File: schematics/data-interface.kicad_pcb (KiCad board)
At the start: 4 copper layers, 30.1 x 69.9 mm, 18 parts, among them J2 USB_A, J5 Trigger Button Input Connector, Q1 2SC945, Q2 2SC945, Q3 2SC945, SW3 SW_Push, SW4 SW_DIP_x08

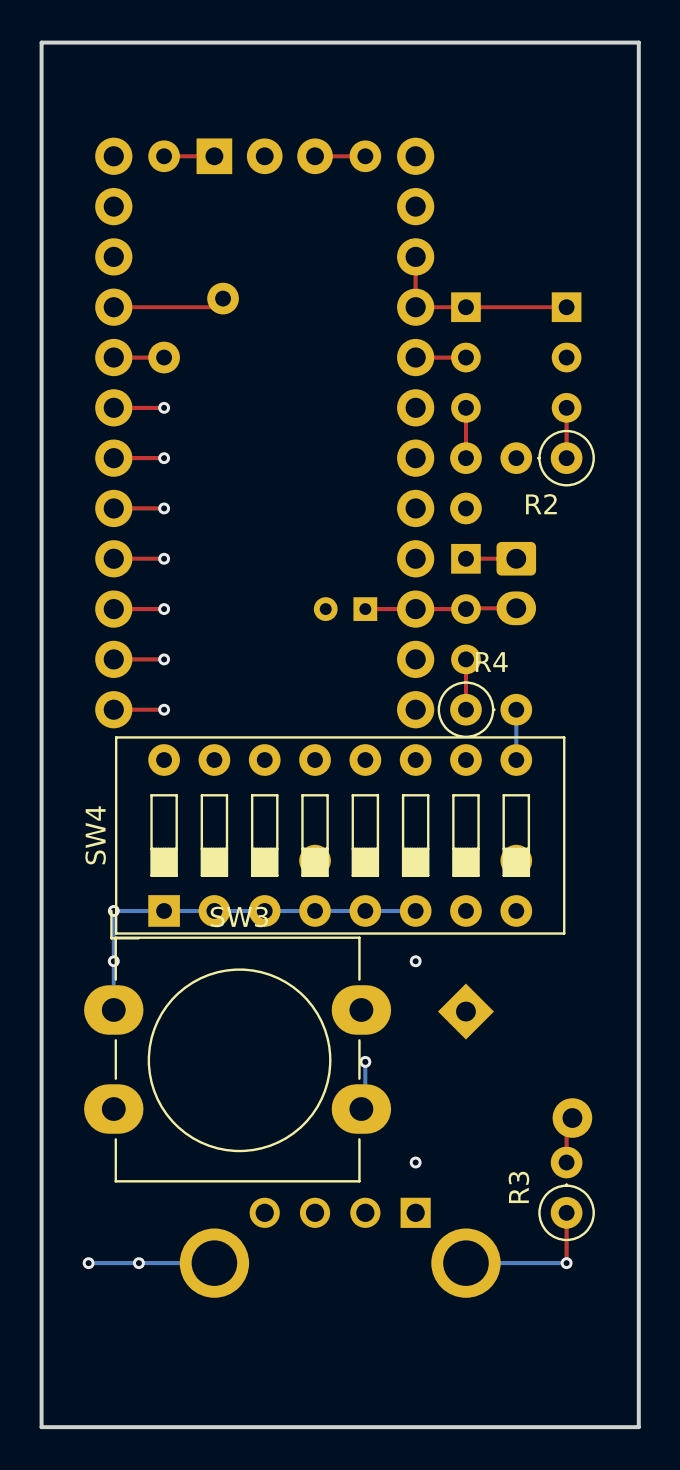
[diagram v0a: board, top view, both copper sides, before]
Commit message: Fixed minor errors in schematics
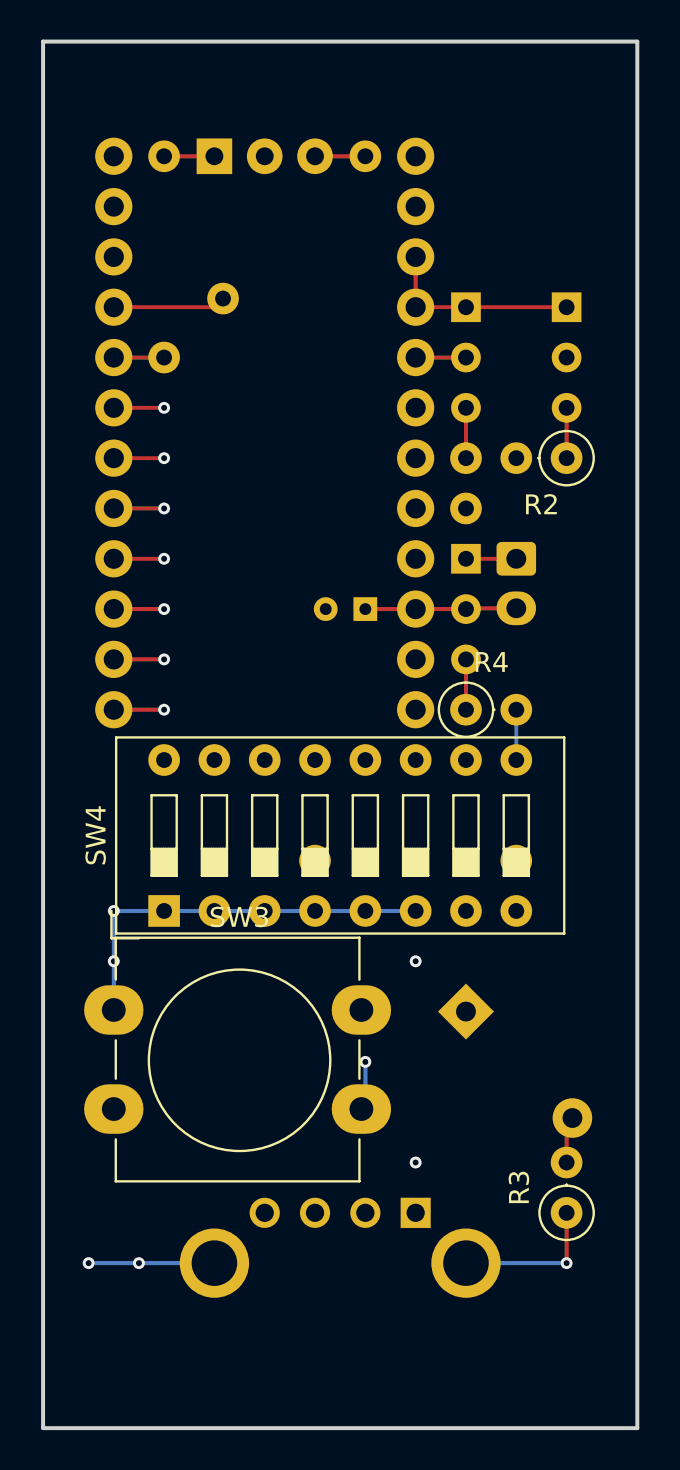
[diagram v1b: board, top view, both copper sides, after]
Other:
- board size 30.1 x 69.9 mm -> 30 x 70 mm
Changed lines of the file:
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@@
 	)
 	(gr_rect
-		(start 134.83 70.345)
-		(end 164.98 140.245)
+		(start 134.905 70.295)
+		(end 164.905 140.295)
 		(stroke
 			(width 0.2)
@@
 		(layer "Edge.Cuts")
 	)
+	(gr_text_box "Example layout for a 2.54mm 10x24 (30x70mm) protoboard."
+		(start 133.395 54.495)
+		(end 166.415 64.655)
+		(layer "Cmts.User")
+		(effects
+			(font
+				(size 1.5 1.5)
+				(thickness 0.3)
+				(bold yes)
+			)
+			(justify left top)
+		)
+		(border yes)
+		(stroke
+			(width 0.2)
+			(type solid)
+		)
+	)
 	(segment
